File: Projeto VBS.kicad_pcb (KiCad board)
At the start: 2 copper layers, 120 x 120 mm, 7 parts, among them J1 Screw_Terminal_01x02, J1_tx/rx1 Conn_01x03_Pin, J2_fins_de_curso1 Conn_01x03_Pin, J3 Conn_01x03_Pin, J4 Conn_01x06_Pin

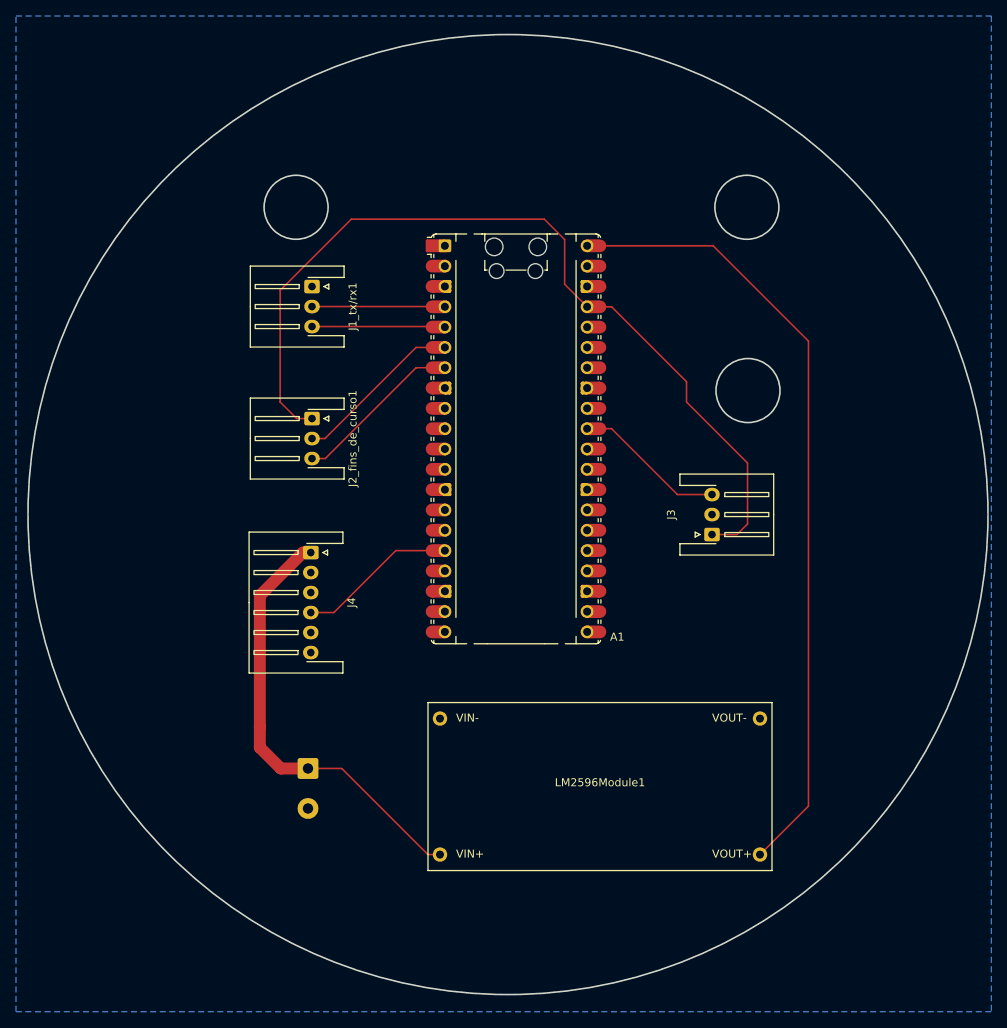
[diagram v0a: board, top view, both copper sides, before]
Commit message: acho que esta pronto
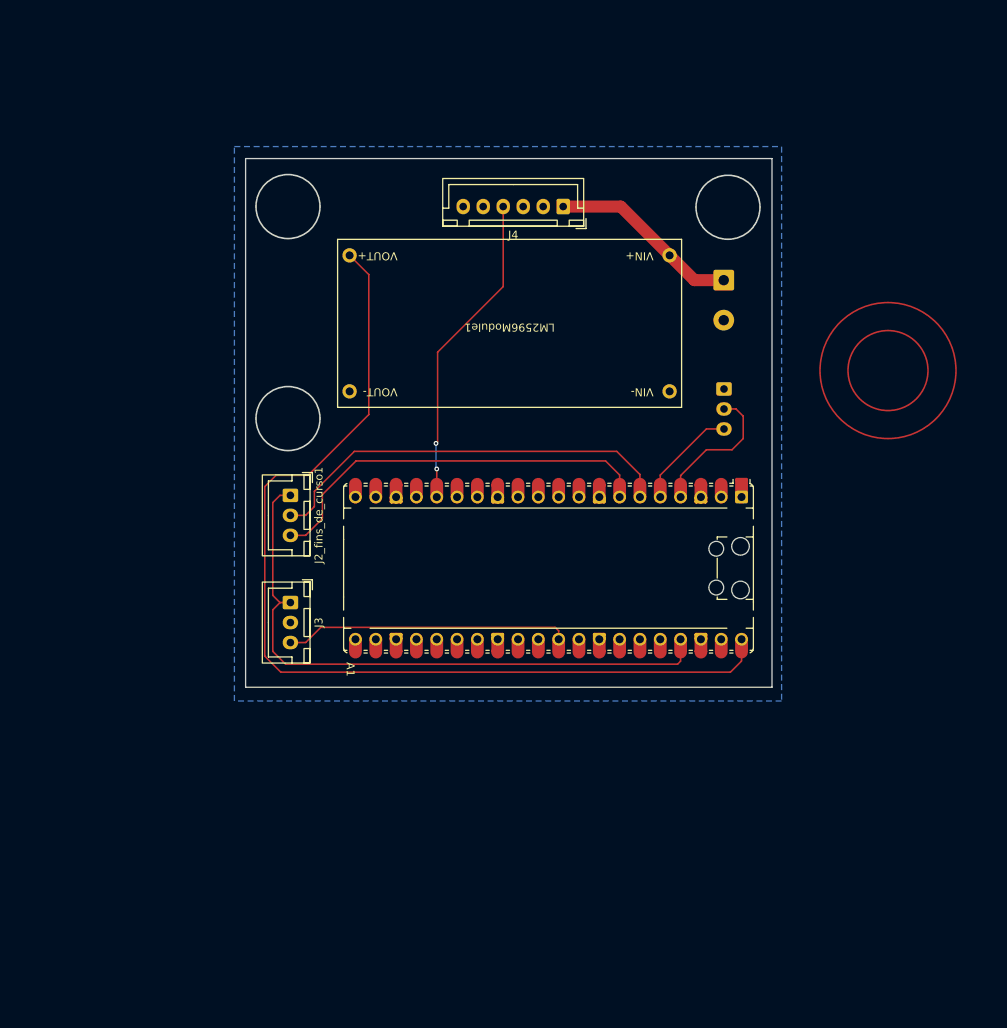
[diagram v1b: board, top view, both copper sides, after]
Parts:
- J1_tx/rx1: footprint Connector_JST:JST_XH_S3B-XH-A-1_1x03_P2.50mm_Horizontal -> Connector_JST:JST_XH_B3B-XH-A_1x03_P2.50mm_Vertical; moved to B.Cu
- J2_fins_de_curso1, J3: footprint Connector_JST:JST_XH_S3B-XH-A-1_1x03_P2.50mm_Horizontal -> Connector_JST:JST_XH_B3B-XH-A_1x03_P2.50mm_Vertical
- J4: footprint Connector_JST:JST_XH_S6B-XH-A-1_1x06_P2.50mm_Horizontal -> Connector_JST:JST_XH_B6B-XH-A_1x06_P2.50mm_Vertical
- moved J1 80.2 mm to (152.0, 76.2)
- moved LM2596Module1 59.0 mm to (125.2, 81.6), turned to 180 degrees
- moved J4 53.5 mm to (131.9, 67.0), turned to 180 degrees
- moved J3 53.4 mm to (97.8, 116.5), turned to -90 degrees
- moved J1_tx/rx1 53.1 mm to (152.0, 89.8)
- moved A1 16.7 mm to (130.1, 112.2), turned to -90 degrees
- moved J2_fins_de_curso1 9.97 mm to (97.8, 103.1)
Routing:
- net Net-(A1-3V3_EN): track 110.1 -> 77.7 mm
- net Net-(J1-Pin_1): track 55.6 -> 23.9 mm
- net Net-(A1-GPIO4): track 20.5 -> 52.1 mm
- net Net-(A1-GPIO5): track 20.5 -> 50.2 mm
- net Net-(A1-VBUS): track 98.5 -> 121.7 mm
- net Net-(A1-GPIO12): track 19.2 -> 39.8 mm, vias 0 -> 2
- net Net-(A1-GPIO26_ADC0): track 18.2 -> 35.6 mm
- net Net-(A1-GPIO3): track 15.8 -> 12.3 mm
- net Net-(A1-GPIO2): track 15.8 -> 17.2 mm
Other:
- board size 120 x 120 mm -> 65.8 x 66.1 mm
